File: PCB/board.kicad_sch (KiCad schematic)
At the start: 5 parts, among them SW1 SW_Push, SW2 SW_Push, SW3 SW_Push, SW4 SW_Push, U1 MOUDLE-SEEEDUINO-XIAO

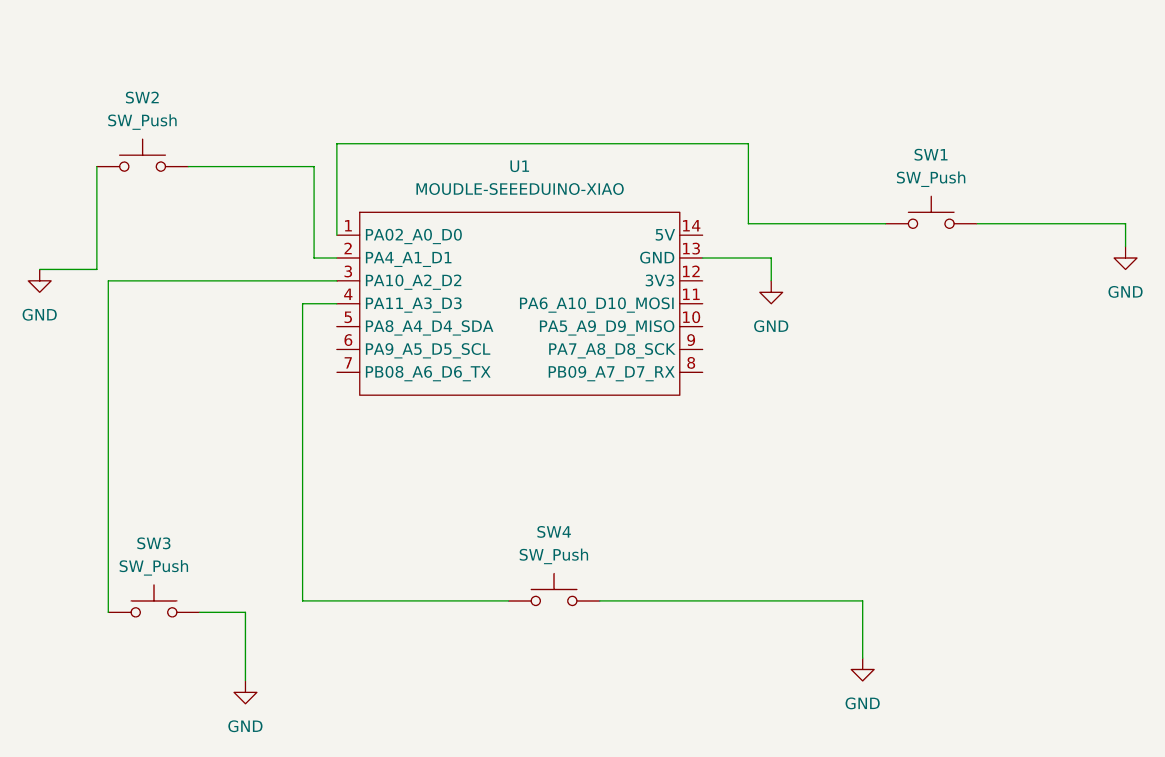
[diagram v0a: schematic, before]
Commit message: Add firmware
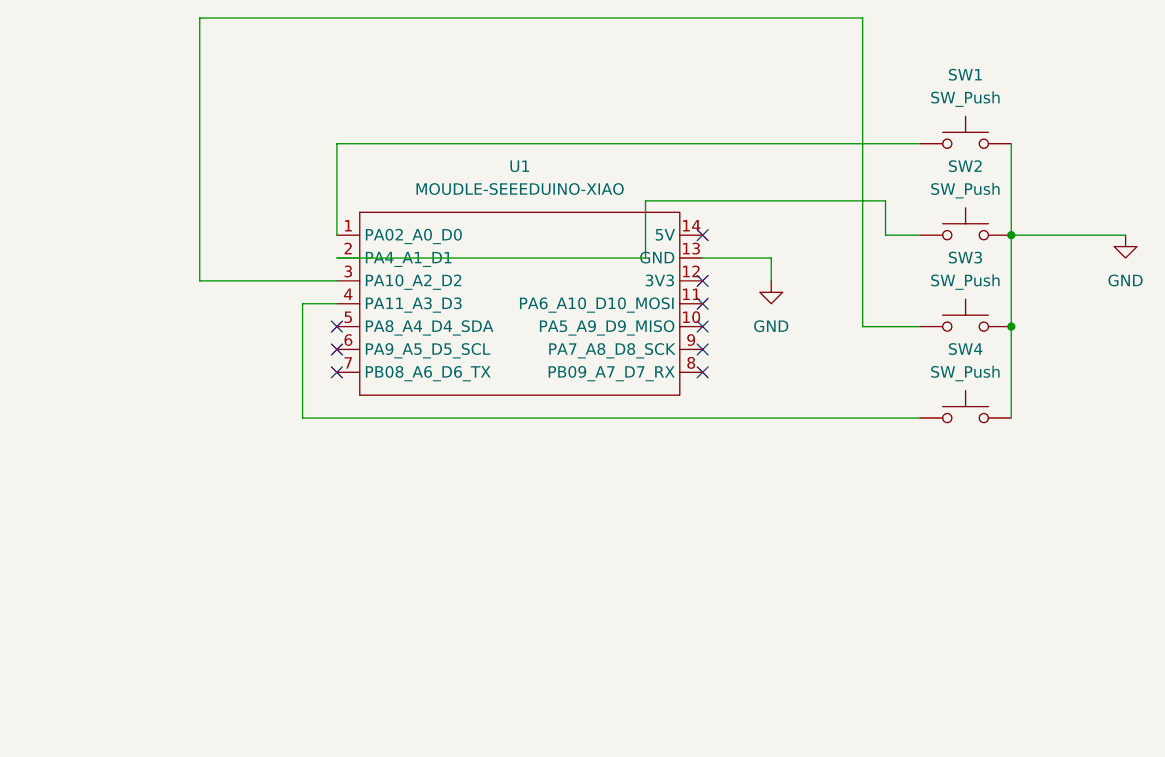
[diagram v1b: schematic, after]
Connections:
- net GND: now also SW2.2; no longer SW2.1
- net at U1.2 (PA4_A1_D1): now also SW2.1; no longer SW2.2
- no-connect marks 0 -> 9
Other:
- moved on the sheet: SW1, SW2, SW3, SW4
